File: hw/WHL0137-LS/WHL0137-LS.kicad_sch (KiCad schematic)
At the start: 0 parts

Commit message: Initial schematic
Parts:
- added D73: LED_Small, LED_SMD:LED_0805_2012Metric, symbol Device:LED_Small
- added J1: Conn_01x05, Connector_JST:JST_EH_S5B-EH_1x05_P2.50mm_Horizontal, symbol Connector_Generic:Conn_01x05
- added R5: 510, Resistor_SMD:R_0805_2012Metric, symbol Device:R
- added TP1, TP2: TestPoint, TestPoint:TestPoint_Pad_D2.5mm, symbol Connector:TestPoint
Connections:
- new net: D73.2 (A), R5.2
- new net +5V: J1.1 (Pin_1), R5.1, TP1.1
- new net GND: D73.1 (K), J1.5 (Pin_5), TP2.1
- new net inner_LED_ring/SCL: J1.3 (Pin_3)
- new net inner_LED_ring/SDA: J1.2 (Pin_2)
- new net inner_LED_ring/SDB: J1.4 (Pin_4)
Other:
- added sheet inner_LED_ring (LED_ring.kicad_sch)
- added sheet outer_LED_ring (LED_ring.kicad_sch)
- title: (none) -> WHL0137-LS

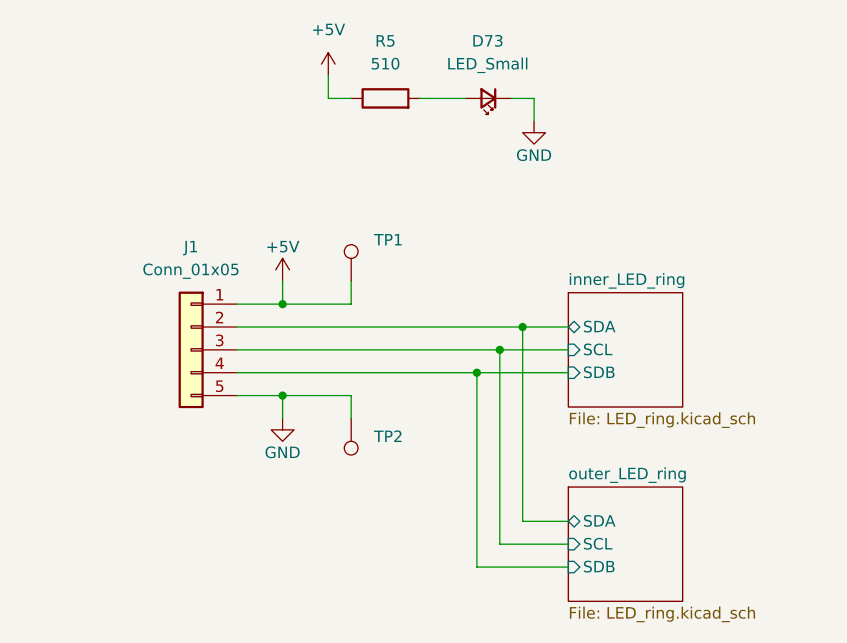
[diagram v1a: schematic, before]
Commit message: Some layout
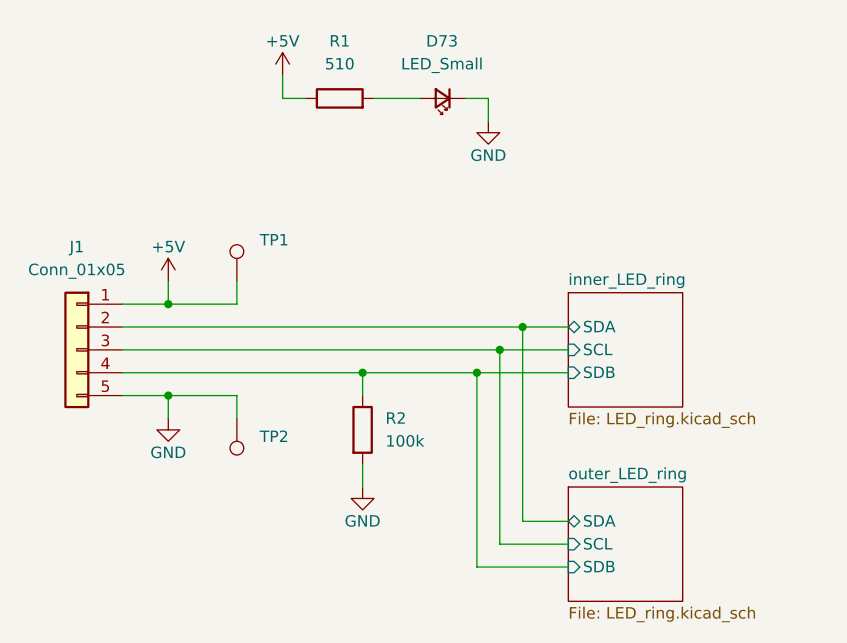
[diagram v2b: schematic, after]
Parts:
- added R2: 100k, Resistor_SMD:R_0805_2012Metric, symbol Device:R
- renumbered R5 to R1
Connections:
- net GND: now also R2.2
- net inner_LED_ring/SDB: now also R2.1
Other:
- moved on the sheet: D73, J1, R1, TP1, TP2
